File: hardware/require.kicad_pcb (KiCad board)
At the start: 6 copper layers, 48 x 28.6 mm, 165 parts, among them J800 Molex 105164-0001, J801 Molex 105164-0001, U100 RK3308, U200 SY8089AAC, U220 PAM2305CGFADJ, U230 PAM2305CGFADJ, U250 SY8089AAC, U260 NCP707CMX180TCG, U300 DDR3_FBGA96, U400 EMMC_BGA_153, U500 ap6255, U830 ATECC608A-MAHDA, Y100 24MHz,12pF,10ppm, Y520 37.4MHz,9pF,10ppm

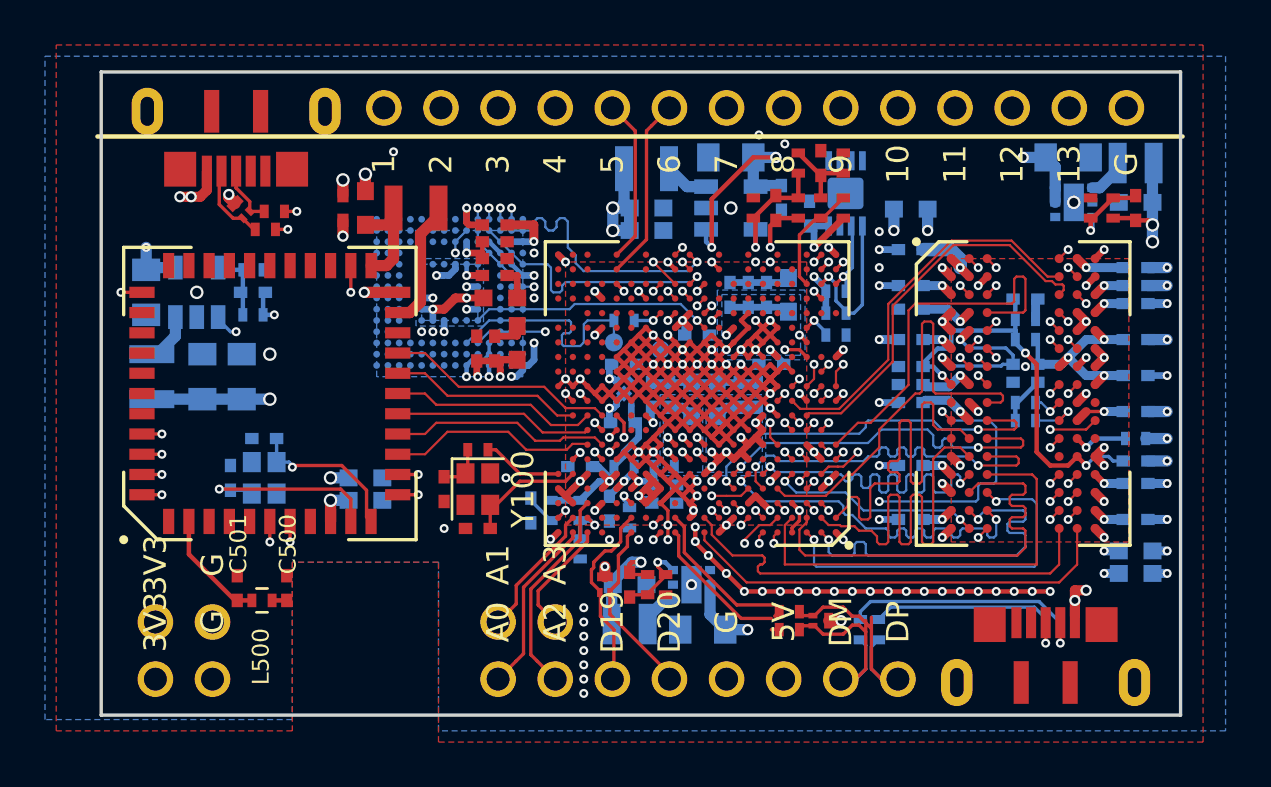
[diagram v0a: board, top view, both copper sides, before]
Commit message: prepare gerber and drill
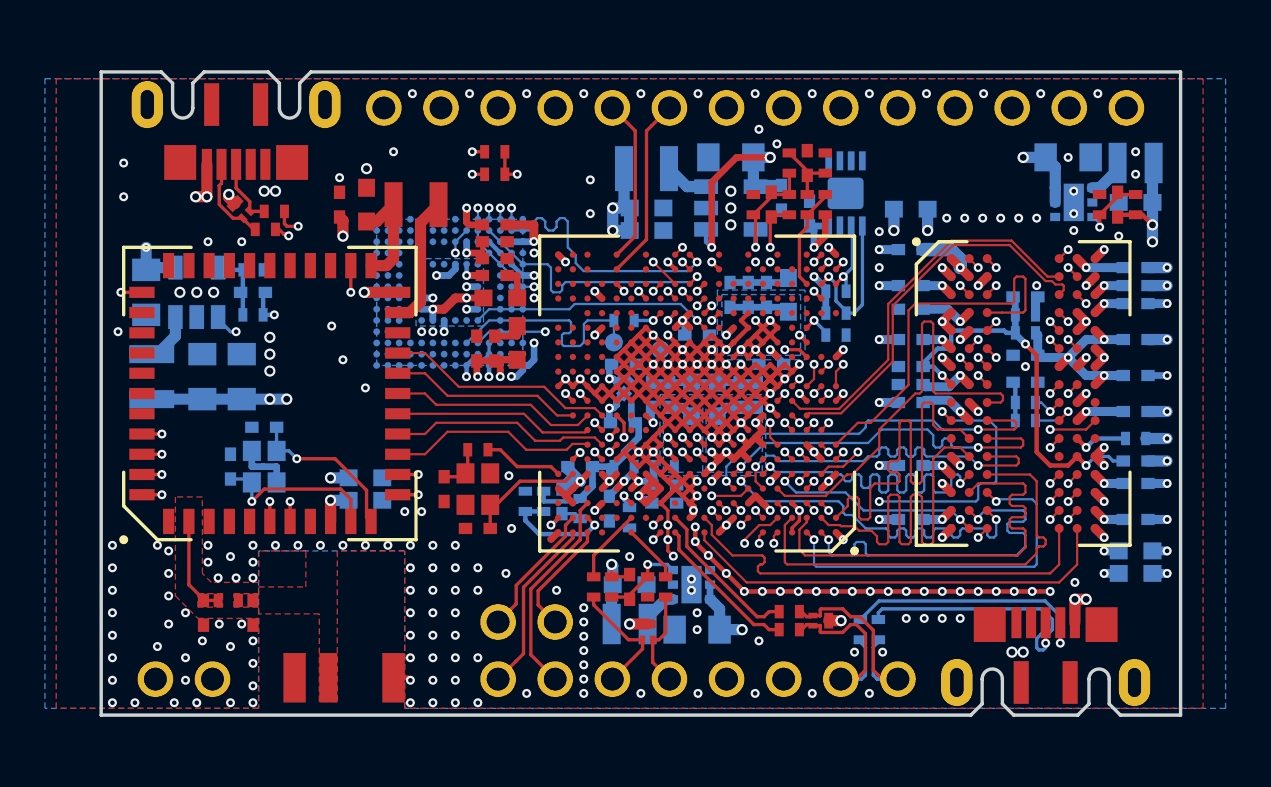
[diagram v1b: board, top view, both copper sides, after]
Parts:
- removed the LP1 at (43.5, 75.2)
- removed LP16: 3V3, require:OVAL_PIN
- removed LP18: 5V, require:OVAL_PIN
- added ANT1: ANT_LA52H2450_5500_A28, require:LA52H2450_5500_A28, F.Cu at (49.3, 77.6)
- added LP8: 5V, require:OVAL_PIN, F.Cu at (68.8, 77.7)
- added R820: 22R, require:R_0402, F.Cu at (60.4, 73.6)
- added R821: 22R, require:R_0402, F.Cu at (63.6, 73.6)
- added R840: 10k, require:R_0402, F.Cu at (56.0, 54.2)
- added R841: 10k, require:R_0402, F.Cu at (56.0, 55.2)
- F229, F269: footprint Inductors_SMD:L_0402 -> require:L_0402
- Y100, Y520: footprint Crystals:Crystal_SMD_2016-4pin_2.0x1.6mm -> require:Crystal_SMD_2016-4pin_2.0x1.6mm
- moved R701 3.23 mm to (57.4, 69.8), turned to 90 degrees
- moved D820 2.83 mm to (62.8, 75.6)
- moved C500 1.86 mm to (45.2, 74.8), turned to 270 degrees
- moved C501 1.86 mm to (43.0, 74.8), turned to 270 degrees
- moved R700 1.68 mm to (58.2, 69.8)
- moved R222 1.60 mm to (61.2, 73.6)
- moved L500 1.50 mm to (44.1, 74.2)
- moved C110 1.44 mm to (59.0, 69.8), turned to 90 degrees
- moved R110 1.30 mm to (59.8, 70.1)
- moved R232 1.01 mm to (84.5, 56.6)
- moved C232 0.81 mm to (83.7, 56.6)
- moved R213 0.81 mm to (70.7, 56.6)
- moved R223 0.81 mm to (62.8, 73.6)
- moved R211 0.80 mm to (70.7, 54.8)
- moved R212 0.62 mm to (69.9, 56.6)
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- renumbered LP17 to LP1, LP14 to LP2, LP2 to LP3, LP3 to LP31, LP5 to LP41, LP11 to LP5, LP12 to LP6, RP2 to RP1, RP11 to RP10, RP12 to RP11, RP13 to RP12, RP14 to RP13, RP18 to RP14, RP3 to RP2, RP4 to RP3, RP5 to RP4, RP6 to RP5, RP7 to RP6, RP8 to RP7, RP9 to RP8, RP10 to RP9
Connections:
- net /rk3308-io/USB_HOST_DM renamed /USB_HOST_D1_N
- net /rk3308-io/USB_HOST_DP renamed /USB_HOST_D1_P
- net Net-(C501-Pad1) renamed /wireless/RFOUT
- net Net-(D810-Pad1) renamed /USB_HOST_D2_P
- net Net-(D810-Pad2) renamed /USB_HOST_D2_N
- net Net-(J801-Pad2) renamed /USB_HOST_D3_P
- net Net-(J801-Pad3) renamed /USB_HOST_D3_N
- C500 pad 1: Net-(C500-Pad1) -> GND
- D820 pad 1: /rk3308-io/D19 -> Net-(D820-Pad1)
- D820 pad 2: /rk3308-io/D20 -> Net-(D820-Pad2)
- L500 pad 2: Net-(C500-Pad1) -> GND
- LP5 pad 1: /rk3308-io/D19 -> Net-(D820-Pad1)
- LP6 pad 1: /rk3308-io/D20 -> Net-(D820-Pad2)
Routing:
- net +3V3: track 69.7 -> 76.1 mm, vias 19 -> 22
- net Net-(D820-Pad1): track 0.00 -> 5.47 mm
- net /rk3308-io/D20: track 8.01 -> 2.61 mm
- net /rk3308-io/D19: track 8.52 -> 3.32 mm
- net /rk3308-io/D2: track 23.0 -> 27.5 mm, vias 2 -> 3
- net Net-(D820-Pad2): track 0.00 -> 4.36 mm
- net /rk3308-io/A4: track 2.00 -> 5.18 mm
- net /rk3308-io/BT_WAKE_HOST: track 19.8 -> 18.0 mm
- net /rk3308-io/HOST_WAKE_BT: track 19.4 -> 17.6 mm
- net /USB_HOST_D3_N: track 9.88 -> 11.6 mm
- net +1V0L: track 9.15 -> 7.98 mm
- net +1V8: track 9.54 -> 10.6 mm
- net /rk3308-io/D1: track 16.8 -> 17.7 mm, vias 1 -> 2
- net Net-(C520-Pad1): track 8.56 -> 7.66 mm
- net /USB_OTG_D_N: track 28.3 -> 29.0 mm
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- added copper zone on F.Cu, net /wireless/RFOUT
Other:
- outline, holes or cut-outs redrawn
- net class Default: trace_width 0.2 -> 0.15
- board text added: "2.4G/5G 802.11ac Wifi + Bluetooth 4.1"
- board text added: "3V3"
- board text added: "512MB DDR3"
- board text added: "5V"
- board text added: "A0"
- board text added: "A1"
- board text added: "A2"
- board text added: "A3"
- board text added: "CK0"
- board text added: "CK2"
- board text added: "CS0"
- board text added: "CS2"
- board text added: "CTS0"
- board text added: "CTS1"
- board text added: "D+"
- board text added: "D-"
- board text added: "D1"
- board text added: "D10"
- board text added: "D11"
- board text added: "D12"
- board text added: "D13"
- board text added: "D2"
- board text added: "D3"
- board text added: "D4"
- board text added: "D5"
- board text added: "D6"
- board text added: "D7"
- board text added: "D8"
- board text added: "D9"
- board text added: "GND"
- board text added: "GPIO0_B6"
- board text added: "GPIO0_B7"
- board text added: "GPIO0_C0"
- board text added: "GPIO1_C6"
- board text added: "GPIO1_C7"
- board text added: "GPIO1_D0"
- board text added: "GPIO1_D1"
- board text added: "GPIO2_A0"
- board text added: "GPIO2_A1"
- board text added: "GPIO2_A2"
- board text added: "GPIO2_A3"
- board text added: "GPIO3_B4"
- board text added: "GPIO3_B5"
- board text added: "GPIO4_D2"
- board text added: "GPIO4_D3"
- board text added: "MI0"
- board text added: "MI2"
- board text added: "MO0"
- board text added: "MO2"
- board text added: "On-board 8G/16G eMMC (bottom side)"
- board text added: "On-board Microchip CryptoAuth chip for secure authentication (bottom side)"
- board text added: "PWM1"
- board text added: "PWM2"
- board text added: "PWM3"
- board text added: "RTS0"
- board text added: "RTS1"
- board text added: "RX0"
- board text added: "RX1"
- board text added: "RX2"
- board text added: "RX2/TCK"
- board text added: "RX3"
- board text added: "Rockchip RK3308, Quad-Core A35"
- board text added: "SCL0"
- board text added: "SCL2"
- board text added: "SCL3"
- board text added: "SDA0"
- board text added: "SDA2"
- board text added: "SDA3"
- board text added: "TX0"
- board text added: "TX1"
- board text added: "TX2"
- board text added: "TX2/TMS"
- board text added: "TX3"
- board text added: "USB Device & Power"
- board text added: "USB Host"
- board text added: "chip antenna"
